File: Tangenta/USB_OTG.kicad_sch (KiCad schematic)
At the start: 4 parts, among them J11 TYPEC-304-ACP16, U10 TUSB321RWBR, U11 AOZ1353DI-01, U9 PUSB2X4Y-N

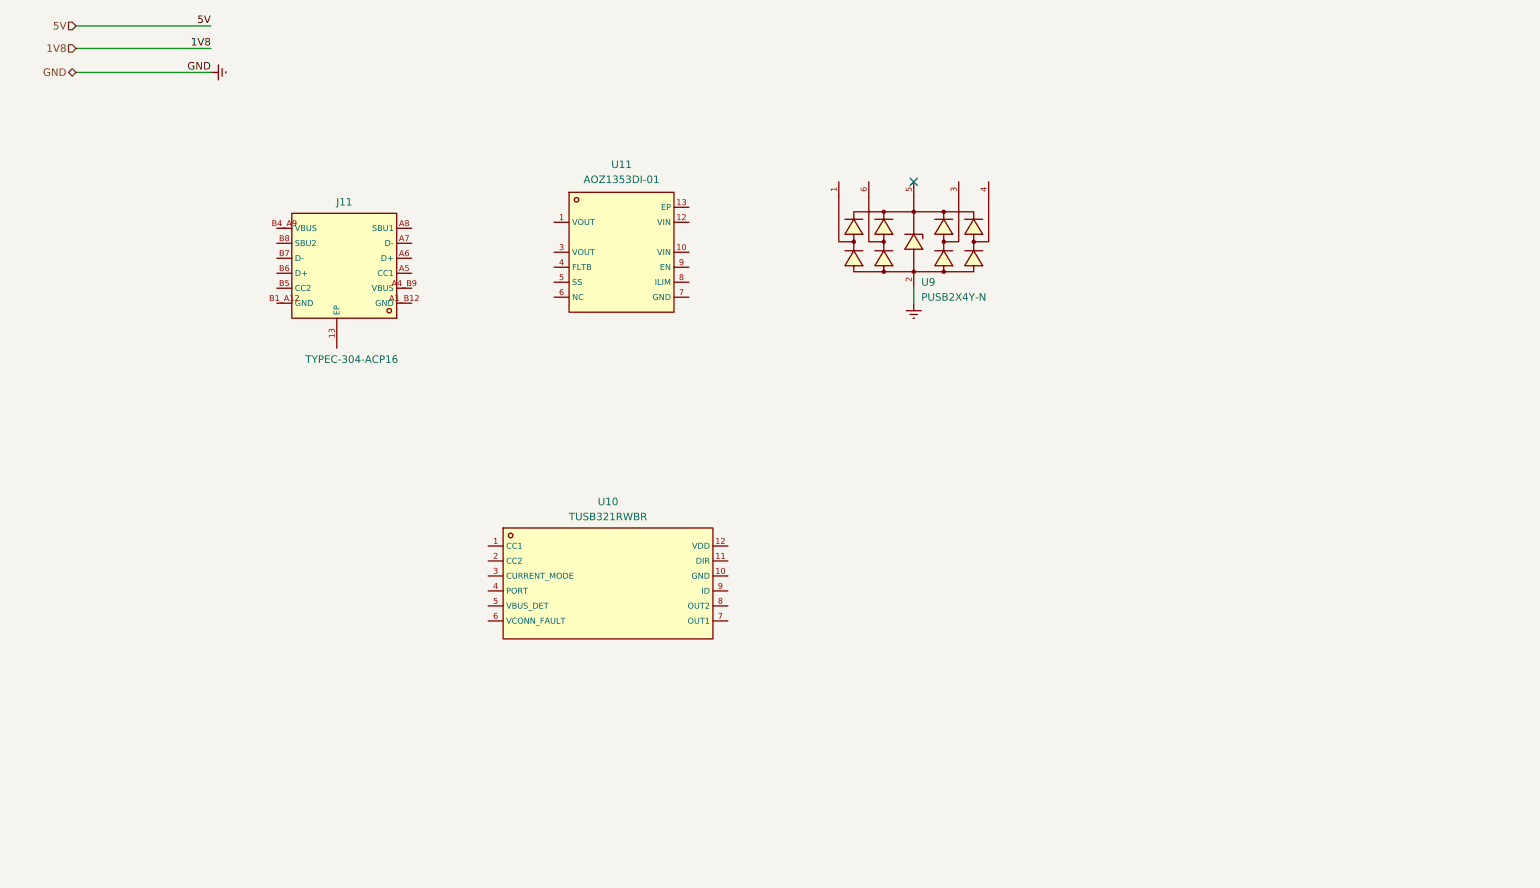
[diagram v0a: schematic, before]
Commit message: USB DualRole in progress...
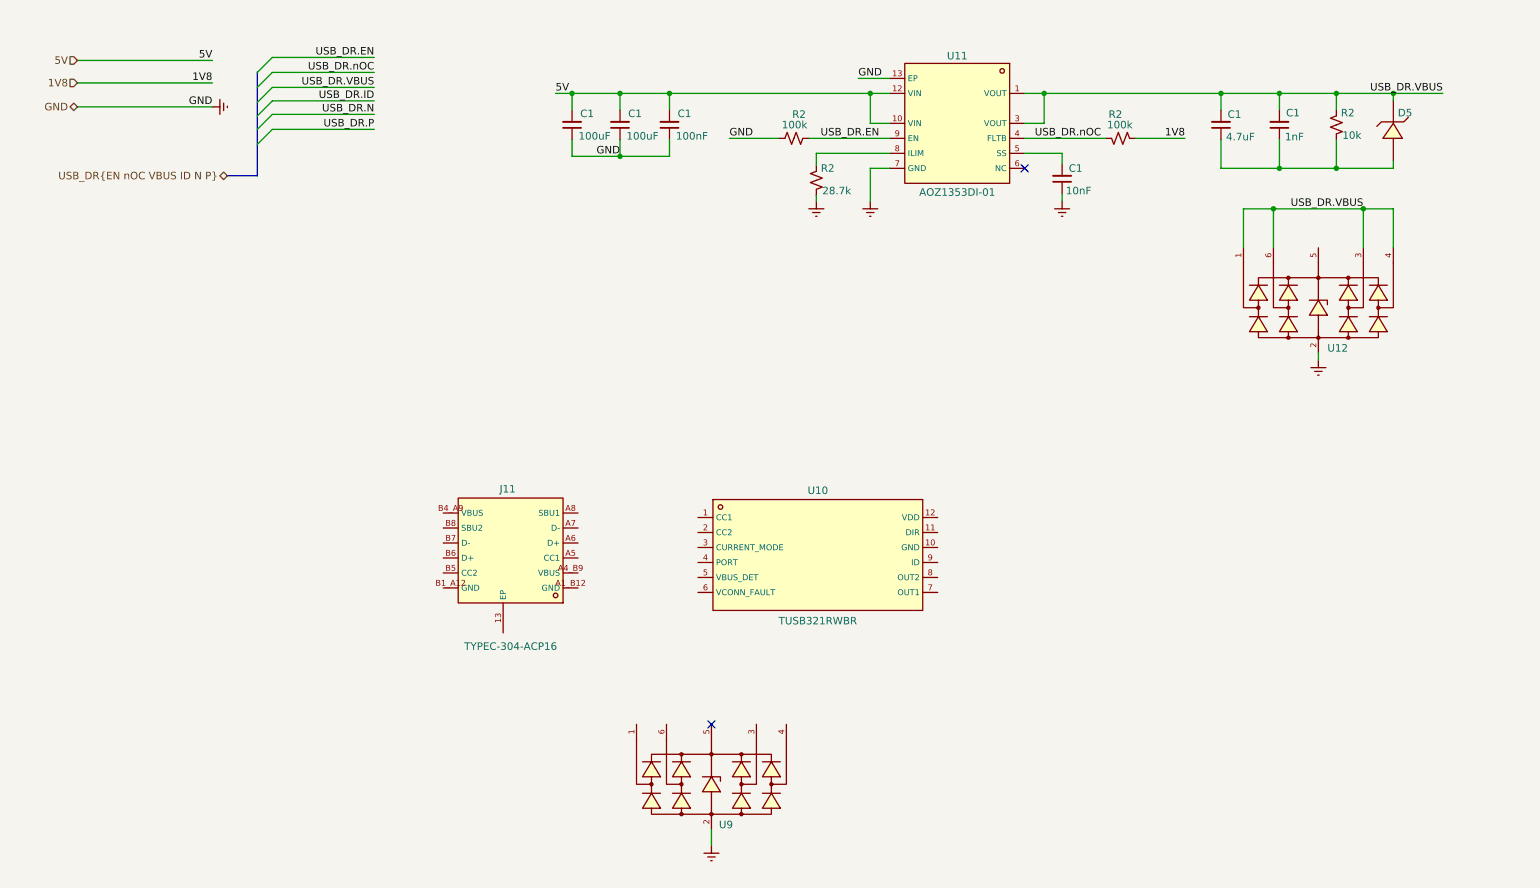
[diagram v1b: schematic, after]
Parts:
- added C1 (x2): 100uF, Capacitor_SMD:C_0402_1005Metric, symbol Device:C_Small
- added C1: 1nF, Capacitor_SMD:C_0402_1005Metric, symbol Device:C_Small
- added C1: 10nF, Capacitor_SMD:C_0402_1005Metric, symbol Device:C_Small
- added C1: 100nF, Capacitor_SMD:C_0402_1005Metric, symbol Device:C_Small
- added C1: 4.7uF, Capacitor_SMD:C_0402_1005Metric, symbol Device:C_Small
- added D5: BZT52C6V2S-7-F, BZT52C6V2S-7-F:BZT52C6V2S-7-F, symbol BZT52C6V2S-7-F:BZT52C6V2S-7-F
- added R2 (x2): 100k, Resistor_SMD:R_0402_1005Metric, symbol Device:R_Small_US
- added R2: 10k, Resistor_SMD:R_0402_1005Metric, symbol Device:R_Small_US
- added R2: 28.7k, Resistor_SMD:R_0402_1005Metric, symbol Device:R_Small_US
- added U12: PUSB2X4Y-N, USB_ESD:USB_ESD, symbol USB_ESD:PUSB2X4Y-N
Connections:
- net 1V8: now also R2.1
- net 5V: now also U11.10 (VIN), U11.12 (VIN), C1.2, C1.2, C1.2
- net GNDREF: now also U11.13 (EP), U11.7 (GND), C1.1, C1.1, C1.1, C1.1, R2.1, R2.1, U12.2 (GND)
- net USB_DR.VBUS: now reaches U11.1 (VOUT)
- net USB_DR.VBUS: now also U11.3 (VOUT), C1.2, C1.2, D5.1 (K), R2.2, U12.1, U12.3, U12.4, U12.6
- net USB_DR.nOC: now reaches U11.4 (FLTB)
- net USB_DR.nOC: now also R2.2
- net at U11.5 (SS): now also C1.2
- net at U11.8 (ILIM): now also R2.2
- net USB_DR.EN: now reaches U11.9 (EN)
- net USB_DR.EN: now also R2.2
- new net: C1.1, C1.1, D5.2 (A), R2.1
- no-connect marks 1 -> 2
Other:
- moved on the sheet: J11, U10, U11, U9

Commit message: Current progress...
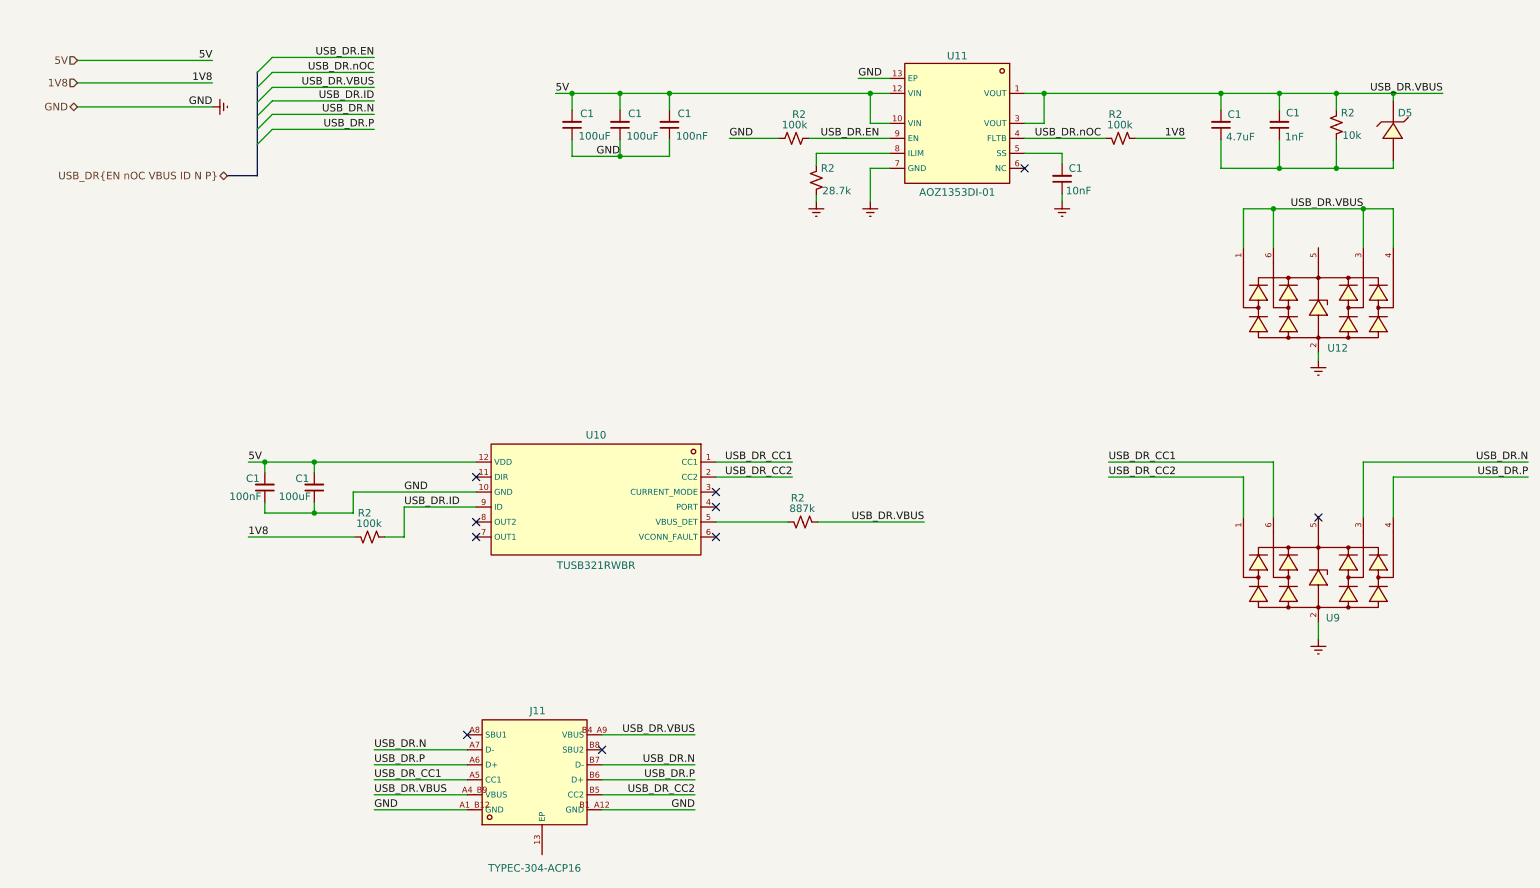
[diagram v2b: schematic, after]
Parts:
- added C1: 100nF, Capacitor_SMD:C_0402_1005Metric, symbol Device:C_Small
- added C1: 100uF, Capacitor_SMD:C_0402_1005Metric, symbol Device:C_Small
- added R2: 887k, Resistor_SMD:R_0402_1005Metric, symbol Device:R_Small_US
- added R2: 100k, Resistor_SMD:R_0402_1005Metric, symbol Device:R_Small_US
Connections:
- net 1V8: now also R2.2
- net 5V: now also U10.12 (VDD), C1.2, C1.2
- net GNDREF: now also J11.A1_B12 (GND), J11.B1_A12 (GND), U10.10 (GND), C1.1, C1.1
- net USB_DR.ID: now also U10.9 (ID), R2.1
- net USB_DR.N: now also J11.A7 (D-), J11.B7 (D-), U9.3
- net USB_DR.P: now also J11.A6 (D+), J11.B6 (D+), U9.4
- net USB_DR.VBUS: now also J11.A4_B9 (VBUS), J11.B4_A9 (VBUS), R2.1
- net USB_DR_CC1: now reaches J11.A5 (CC1)
- net USB_DR_CC1: now also U10.1 (CC1), U9.6
- net USB_DR_CC2: now reaches J11.B5 (CC2)
- net USB_DR_CC2: now also U10.2 (CC2), U9.1
- net at U10.5 (VBUS_DET): now also R2.2
- no-connect marks 2 -> 10
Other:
- moved on the sheet: J11, U10, U9

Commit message: USB DR schematic done.
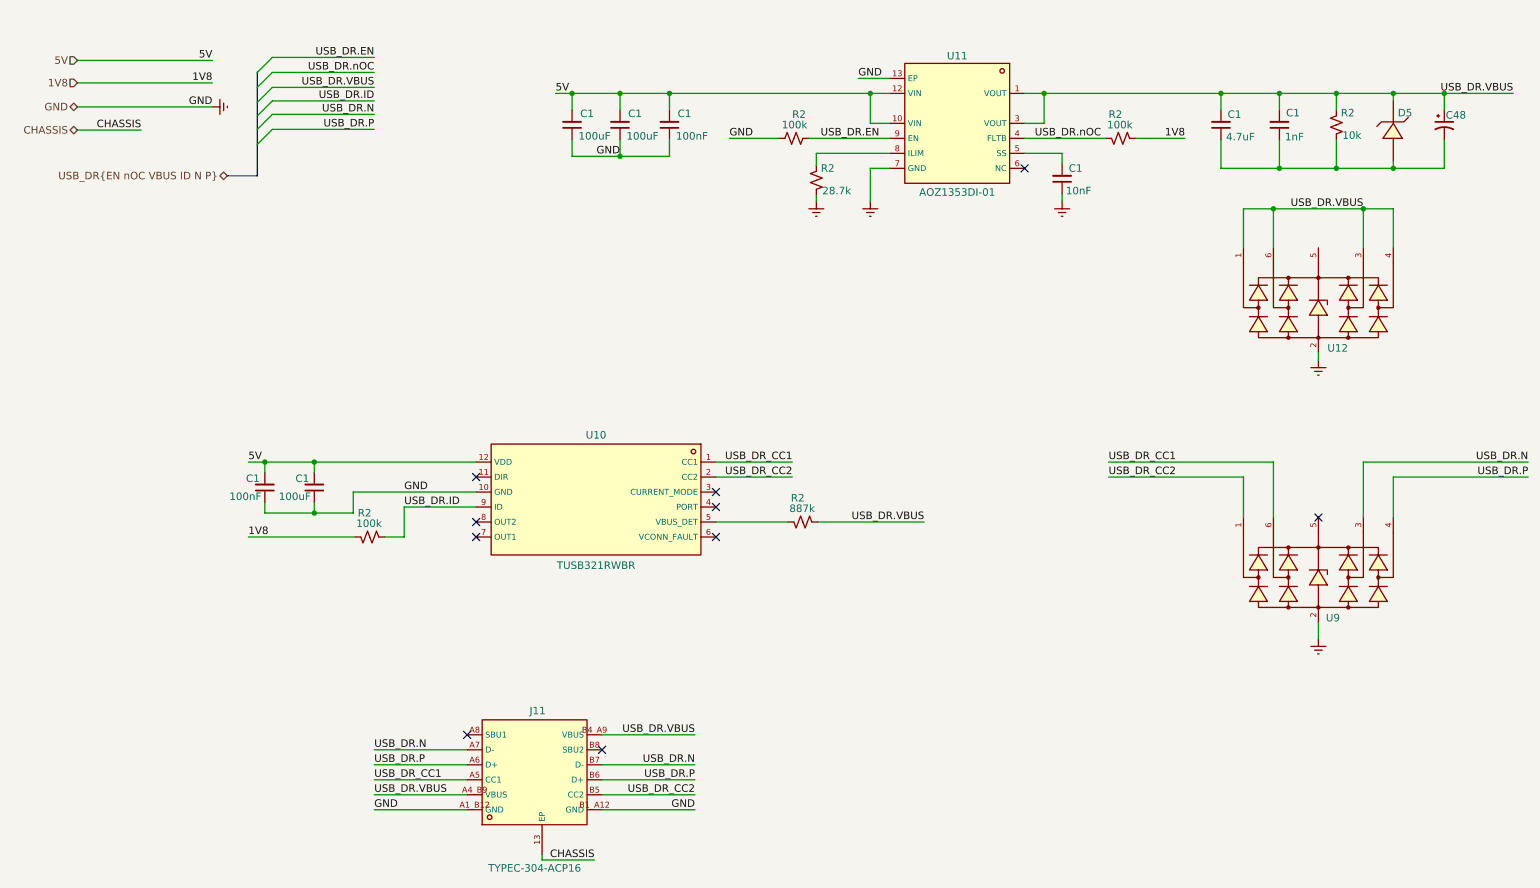
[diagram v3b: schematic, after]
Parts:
- added C48: 16CE47FSS, CAP_L5:CAP_L5, symbol CAP_L5:16CE47FSS
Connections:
- net USB_DR.VBUS: now also C48.1
- net CHASSIS: now reaches J11.13 (EP)
- net at C1.1, C1.1, D5.2 (A)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: now also C48.2
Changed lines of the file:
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@@
   (junction (at 229.87 31.242) (diameter 0) (color 0 0 0 0)
   )
+  (junction (at 259.08 43.942) (diameter 0) (color 0 0 0 0)
+  )
   (junction (at 67.818 93.726) (diameter 0) (color 0 0 0 0)
   )
@@
   )
   (junction (at 249.428 31.242) (diameter 0) (color 0 0 0 0)
+  )
+  (junction (at 267.716 31.242) (diameter 0) (color 0 0 0 0)
   )
   (junction (at 254 50.8) (diameter 0) (color 0 0 0 0)
@@
     (stroke (width 0) (type default))
   )
+  (wire (pts (xy 36.068 37.465) (xy 46.863 37.465))
+    (stroke (width 0) (type default))
+  )
   (wire (pts (xy 173.736 38.862) (xy 160.02 38.862))
     (stroke (width 0) (type default))
@@
     (stroke (width 0) (type default))
   )
+  (wire (pts (xy 114.808 160.274) (xy 114.808 161.163))
+    (stroke (width 0) (type default))
+  )
   (wire (pts (xy 229.87 43.942) (xy 229.87 39.116))
     (stroke (width 0) (type default))
@@
     (stroke (width 0) (type default))
   )
+  (wire (pts (xy 267.716 31.242) (xy 267.716 34.036))
+    (stroke (width 0) (type default))
+  )
   (wire (pts (xy 136.398 31.242) (xy 170.434 31.242))
     (stroke (width 0) (type default))
@@
     (stroke (width 0) (type default))
   )
+  (wire (pts (xy 114.808 161.163) (xy 123.698 161.163))
+    (stroke (width 0) (type default))
+  )
   (wire (pts (xy 239.776 39.116) (xy 239.776 43.942))
     (stroke (width 0) (type default))
@@
     (stroke (width 0) (type default))
   )
+  (wire (pts (xy 267.716 43.942) (xy 259.08 43.942))
+    (stroke (width 0) (type default))
+  )
   (wire (pts (xy 202.946 41.402) (xy 202.946 43.18))
     (stroke (width 0) (type default))
@@
     (stroke (width 0) (type default))
   )
+  (wire (pts (xy 267.716 39.116) (xy 267.716 43.942))
+    (stroke (width 0) (type default))
+  )
   (wire (pts (xy 124.968 139.954) (xy 140.716 139.954))
     (stroke (width 0) (type default))
@@
     (stroke (width 0) (type default))
   )
-  (wire (pts (xy 259.08 31.242) (xy 267.462 31.242))
+  (wire (pts (xy 259.08 31.242) (xy 267.716 31.242))
     (stroke (width 0) (type default))
   )
@@
     (stroke (width 0) (type default))
   )
+  (wire (pts (xy 267.716 31.242) (xy 279.4 31.242))
+    (stroke (width 0) (type default))
+  )
   (bus (pts (xy 66.548 39.878) (xy 66.548 45.212))
     (stroke (width 0) (type default))
@@
     (effects (font (size 1.27 1.27)) (justify left bottom))
   )
+  (label "CHASSIS" (at 123.698 161.163 180) (fields_autoplaced)
+    (effects (font (size 1.27 1.27)) (justify right bottom))
+  )
   (label "USB_DR.VBUS" (at 140.716 139.954 180) (fields_autoplaced)
     (effects (font (size 1.27 1.27)) (justify right bottom))
@@
     (effects (font (size 1.27 1.27)) (justify right bottom))
   )
-  (label "USB_DR.VBUS" (at 267.462 31.242 180) (fields_autoplaced)
+  (label "USB_DR.VBUS" (at 279.4 31.242 180) (fields_autoplaced)
+    (effects (font (size 1.27 1.27)) (justify right bottom))
+  )
+  (label "CHASSIS" (at 46.863 37.465 180) (fields_autoplaced)
     (effects (font (size 1.27 1.27)) (justify right bottom))
   )
@@
   )
   (hierarchical_label "1V8" (shape input) (at 36.068 29.464 180) (fields_autoplaced)
+    (effects (font (size 1.27 1.27)) (justify right))
+  )
+  (hierarchical_label "CHASSIS" (shape bidirectional) (at 36.068 37.465 180) (fields_autoplaced)
     (effects (font (size 1.27 1.27)) (justify right))
   )
@@
         )
       )
+    )
+  )
+  (symbol (lib_id "CAP_L5:16CE47FSS") (at 267.716 36.576 0) (unit 1)
+    (in_bom yes) (on_board yes) (dnp no)
+    (property "Reference" "C48" (at 267.97 34.925 0)
+      (effects (font (size 1.27 1.27)) (justify left))
+    )
+    (property "Value" "16CE47FSS" (at 270.129 37.4142 0)
+      (effects (font (size 1.27 1.27)) (justify left) hide)
+    )
+    (property "Footprint" "CAP_L5:CAP_L5" (at 266.446 54.356 0)
+      (effects (font (size 1.27 1.27) italic) hide)
+    )
+    (property "Datasheet" "https://item.szlcsc.com/245725.html" (at 259.334 52.07 0)
+      (effects (font (size 1.27 1.27)) (justify left) hide)
+    )
+    (property "LCSC" "C242026" (at 263.652 49.784 0)
+      (effects (font (size 1.27 1.27)) hide)
+    )
+    (property "Capacitance" "47uF" (at 272.288 36.83 0)
+      (effects (font (size 1.27 1.27)) hide)
+    )
+    (pin "1")
+    (pin "2")
+    (instances
+      (project "Tangenta"
+        (path "/358d1bcf-7599-4352-8c4d-baa18a5f09e6/b1871a4d-6a35-44e2-a9a2-9a4af684371d"
+          (reference "C48") (unit 1)
+        )
+        (path "/358d1bcf-7599-4352-8c4d-baa18a5f09e6/e56d8c10-557c-47b7-a4d3-5b3b43580080"
+          (reference "C58") (unit 1)
+        )
+      )
